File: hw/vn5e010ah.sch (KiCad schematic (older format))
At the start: 4 parts, among them U1001 VN5E010AH

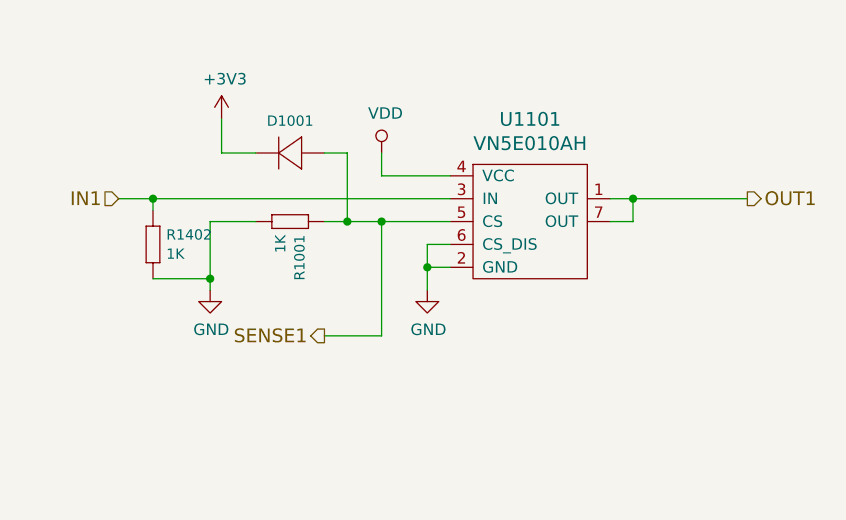
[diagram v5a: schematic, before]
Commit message: new ESB 5.2.0 sent
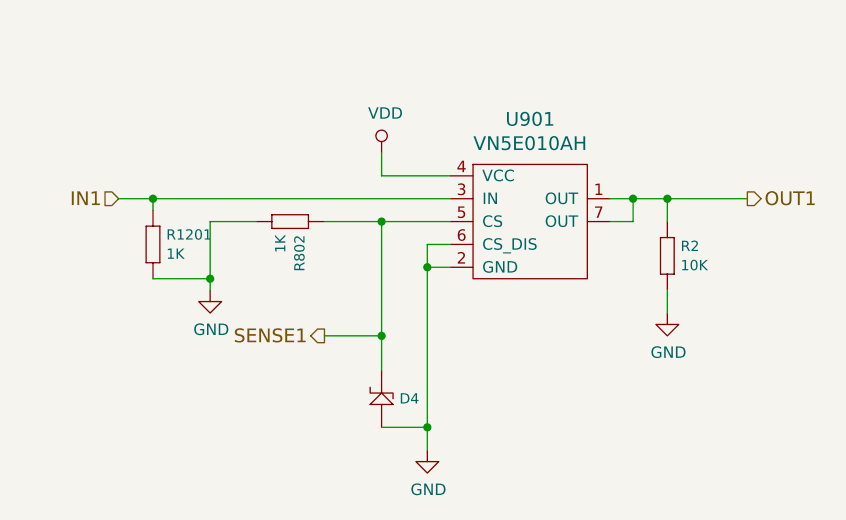
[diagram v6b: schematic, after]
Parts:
- removed D1201: DIODE_RS07J-GS18, usevolt:DO219AB, symbol usevolt:DIODE_RS07J-GS18
- added D3: ZENER_MM3Z3V6T1G, usevolt:SOD-323, symbol usevolt:ZENER_MM3Z3V6T1G
- added R1: 10K, yageo:0603, symbol yageo:10K
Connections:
- net GND: now also D3.2, R1.1 (R1)
- net OUT1: now also R1.2 (R2)
- net SENSE1: now also D3.1
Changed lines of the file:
@@
 $Descr A4 11693 8268
 encoding utf-8
-Sheet 7 12
+Sheet 8 13
 Title ""
 Date ""
@@
 SENSE1
 Wire Wire Line
-	4350 3300 4450 3300
-Wire Wire Line
 	3850 3300 4050 3300
 Wire Wire Line
@@
 AR Path="/5A13680F/59D7E637" Ref="#PWR048"  Part="1"
 AR Path="/5A14370A/59D7E637" Ref="#PWR051"  Part="1"
-F 0 "#PWR045" H 4600 2850 50  0001 C CNN
+F 0 "#PWR039" H 4600 2850 50  0001 C CNN
 F 1 "VDD" H 4617 3173 50  0000 C CNN
 F 2 "" H 4600 3000 50  0000 C CNN
@@
 AR Path="/5A13680F/5A014ACD" Ref="#PWR049"  Part="1"
 AR Path="/5A14370A/5A014ACD" Ref="#PWR052"  Part="1"
-F 0 "#PWR046" H 3850 3350 50  0001 C CNN
+F 0 "#PWR040" H 3850 3350 50  0001 C CNN
 F 1 "GND" H 3855 3427 50  0000 C CNN
 F 2 "" H 3850 3600 50  0000 C CNN
@@
 AR Path="/5A13680F/5A058D94" Ref="R1502"  Part="1"
 AR Path="/5A14370A/5A058D94" Ref="R1602"  Part="1"
-F 0 "R1402" V 3608 3408 45  0000 L CNN
+F 0 "R1201" V 3608 3408 45  0000 L CNN
 F 1 "1K" V 3692 3408 45  0000 L CNN
 F 2 "yageo:0603" H 3630 3500 20  0001 C CNN
@@
 AR Path="/5A1358B0/5A32CF4A" Ref="U1101"  Part="1"
 AR Path="/5A13680F/5A32CF4A" Ref="U1201"  Part="1"
-F 0 "U1101" H 5250 3747 60  0000 C CNN
+F 0 "U901" H 5250 3747 60  0000 C CNN
 F 1 "VN5E010AH" H 5250 3641 60  0000 C CNN
 F 2 "usevolt:HPAK" H 4950 4250 60  0001 C CNN
@@
 L power:GND #PWR044
 U 1 1 5A32CF90
-P 4800 3600
+P 4800 4300
 AR Path="/5A1349CF/5A32CF90" Ref="#PWR044"  Part="1"
 AR Path="/5A14370A/5A32CF90" Ref="#PWR053"  Part="1"
@@
 AR Path="/5A1358B0/5A32CF90" Ref="#PWR047"  Part="1"
 AR Path="/5A13680F/5A32CF90" Ref="#PWR050"  Part="1"
-F 0 "#PWR047" H 4800 3350 50  0001 C CNN
-F 1 "GND" H 4805 3427 50  0000 C CNN
-F 2 "" H 4800 3600 50  0000 C CNN
-F 3 "" H 4800 3600 50  0000 C CNN
-	1    4800 3600
+F 0 "#PWR041" H 4800 4050 50  0001 C CNN
+F 1 "GND" H 4805 4127 50  0000 C CNN
+F 2 "" H 4800 4300 50  0000 C CNN
+F 3 "" H 4800 4300 50  0000 C CNN
+	1    4800 4300
 	1    0    0    -1
 $EndComp
@@
 Connection ~ 4800 3500
 Wire Wire Line
-	5700 3200 6200 3200
+	5700 3200 5850 3200
 Wire Wire Line
 	4600 3300 4900 3300
@@
 	3850 3550 3850 3600
 Wire Wire Line
-	4800 3500 4800 3600
+	4800 3500 4800 4200
 $Comp
 L yageo:1K R?
@@
 AR Path="/5A13680F/5B23824A" Ref="R1101"  Part="1"
 AR Path="/5A14370A/5B23824A" Ref="R1202"  Part="1"
-F 0 "R1001" V 4258 3358 45  0000 L CNN
+F 0 "R802" V 4258 3358 45  0000 L CNN
 F 1 "1K" V 4342 3358 45  0000 L CNN
 F 2 "yageo:0603" H 4280 3450 20  0001 C CNN
@@
 $EndComp
 $Comp
-L usevolt:DIODE_RS07J-GS18 D1201
-U 1 1 5B23844A
-P 4150 3000
-AR Path="/5A14370A/5B23844A" Ref="D1201"  Part="1"
-AR Path="/5A12FF64/5B23844A" Ref="D703"  Part="1"
-AR Path="/5A130D3E/5B23844A" Ref="D801"  Part="1"
-AR Path="/5A1349CF/5B23844A" Ref="D901"  Part="1"
-AR Path="/5A1358B0/5B23844A" Ref="D1001"  Part="1"
-AR Path="/5A13680F/5B23844A" Ref="D1101"  Part="1"
-F 0 "D1001" H 4100 2860 45  0000 C CNN
-F 1 "DIODE_RS07J-GS18" H 4170 2940 45  0001 L BNN
-F 2 "usevolt:DO219AB" H 4180 3150 20  0001 C CNN
-F 3 "http://www.vishay.com/docs/85742/rs07b.pdf" H 4170 3020 60  0001 C CNN
-F 4 "1864882" H 4770 3620 60  0001 C CNN "2nd Source Part Number"
-F 5 "Digi-Key" H 4470 3320 60  0001 C CNN "1st Source"
-F 6 "Farnell" H 4670 3520 60  0001 C CNN "2nd Source"
-F 7 "RS07J-GS18" H 4370 3220 60  0001 C CNN "Manufacturer Part Number"
-F 8 "RS07J-GS18-ND" H 4570 3420 60  0001 C CNN "1st Source Part Number"
-F 9 "Vishay Semiconductor Diodes Division" H 4270 3120 60  0001 C CNN "Manufacturer"
-	1    4150 3000
-	-1   0    0    1
-$EndComp
-$Comp
-L power:+3V3 #PWR0107
-U 1 1 5B23856B
-P 3900 2850
-AR Path="/5A14370A/5B23856B" Ref="#PWR0107"  Part="1"
-AR Path="/5A12FF64/5B23856B" Ref="#PWR0102"  Part="1"
-AR Path="/5A130D3E/5B23856B" Ref="#PWR0103"  Part="1"
-AR Path="/5A1349CF/5B23856B" Ref="#PWR0104"  Part="1"
-AR Path="/5A1358B0/5B23856B" Ref="#PWR0105"  Part="1"
-AR Path="/5A13680F/5B23856B" Ref="#PWR0106"  Part="1"
-F 0 "#PWR0105" H 3900 2700 50  0001 C CNN
-F 1 "+3V3" H 3915 3023 50  0000 C CNN
-F 2 "" H 3900 2850 50  0000 C CNN
-F 3 "" H 3900 2850 50  0000 C CNN
-	1    3900 2850
-	1    0    0    -1
-$EndComp
-Wire Wire Line
-	3900 2850 3900 3000
-Wire Wire Line
-	3900 3000 4050 3000
-Wire Wire Line
-	4350 3000 4450 3000
-Wire Wire Line
-	4450 3000 4450 3300
-Connection ~ 4450 3300
-Wire Wire Line
-	4450 3300 4600 3300
+L yageo:10K R1
+U 1 1 5BA9BFAA
+P 5850 3400
+AR Path="/5A12FF64/5BA9BFAA" Ref="R1"  Part="1"
+AR Path="/5A130D3E/5BA9BFAA" Ref="R2"  Part="1"
+AR Path="/5A1349CF/5BA9BFAA" Ref="R3"  Part="1"
+AR Path="/5A1358B0/5BA9BFAA" Ref="R4"  Part="1"
+F 0 "R2" V 5858 3458 45  0000 L CNN
+F 1 "10K" V 5942 3458 45  0000 L CNN
+F 2 "yageo:0603" H 5880 3550 20  0001 C CNN
+F 3 "" H 5819 3439 60  0001 C CNN
+F 4 "" H 6219 3839 60  0001 C CNN "1st Source Part Number"
+F 5 "Digikey" H 6119 3739 60  0001 C CNN "1st Source"
+F 6 "RC0603FR-0710KL" H 6019 3639 60  0001 C CNN "Manufacturer Part Number"
+F 7 "YAGEO" H 5919 3539 60  0001 C CNN "Manufacturer"
+	1    5850 3400
+	0    1    1    0
+$EndComp
+Wire Wire Line
+	5850 3300 5850 3200
+Connection ~ 5850 3200
+Wire Wire Line
+	5850 3200 6200 3200
+$Comp
+L power:GND #PWR0106
+U 1 1 5BA9C33E
+P 5850 3700
+AR Path="/5A12FF64/5BA9C33E" Ref="#PWR0106"  Part="1"
+AR Path="/5A130D3E/5BA9C33E" Ref="#PWR0107"  Part="1"
+AR Path="/5A1349CF/5BA9C33E" Ref="#PWR0108"  Part="1"
+AR Path="/5A1358B0/5BA9C33E" Ref="#PWR0109"  Part="1"
+F 0 "#PWR0107" H 5850 3450 50  0001 C CNN
+F 1 "GND" H 5855 3527 50  0000 C CNN
+F 2 "" H 5850 3700 50  0000 C CNN
+F 3 "" H 5850 3700 50  0000 C CNN
+	1    5850 3700
+	1    0    0    -1
+$EndComp
+Wire Wire Line
+	5850 3700 5850 3600
+Wire Wire Line
+	4350 3300 4600 3300
+$Comp
+L usevolt:ZENER_MM3Z3V6T1G D3
+U 1 1 5BAABE3C
+P 4600 4000
+AR Path="/5A12FF64/5BAABE3C" Ref="D3"  Part="1"
+AR Path="/5A130D3E/5BAABE3C" Ref="D4"  Part="1"
+AR Path="/5A1349CF/5BAABE3C" Ref="D5"  Part="1"
+AR Path="/5A1358B0/5BAABE3C" Ref="D6"  Part="1"
+F 0 "D4" V 4525 3922 45  0000 R CNN
+F 1 "ZENER_MM3Z3V6T1G" H 4875 4375 45  0001 L BNN
+F 2 "usevolt:SOD-323" H 4575 4375 20  0001 C CNN
+F 3 "http://www.mouser.com/ds/2/308/MM3Z2V4T1-D-269162.pdf" H 4950 4575 60  0001 C CNN
+F 4 "Mouser" H 4920 4320 60  0001 C CNN "1st Source"
+F 5 "MM3Z3V6T1G" H 4820 4220 60  0001 C CNN "Manufacturer Part Number"
+F 6 "863-MM3Z3V6T1G" H 5020 4420 60  0001 C CNN "1st Source Part Number"
+F 7 "ON Semiconductor" H 4875 4475 60  0001 C CNN "Manufacturer"
+	1    4600 4000
+	0    -1   -1   0
+$EndComp
+Wire Wire Line
+	4600 3950 4600 3800
+Connection ~ 4600 3800
+Wire Wire Line
+	4600 4200 4800 4200
+Connection ~ 4800 4200
+Wire Wire Line
+	4800 4200 4800 4300
 $EndSCHEMATC
